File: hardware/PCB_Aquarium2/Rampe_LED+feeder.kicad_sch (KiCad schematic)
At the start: 5 parts, among them J28 Conn_01x03, J29 Conn_01x03, J30 Conn_01x03, J31 Conn_01x03, J32 Conn_01x03

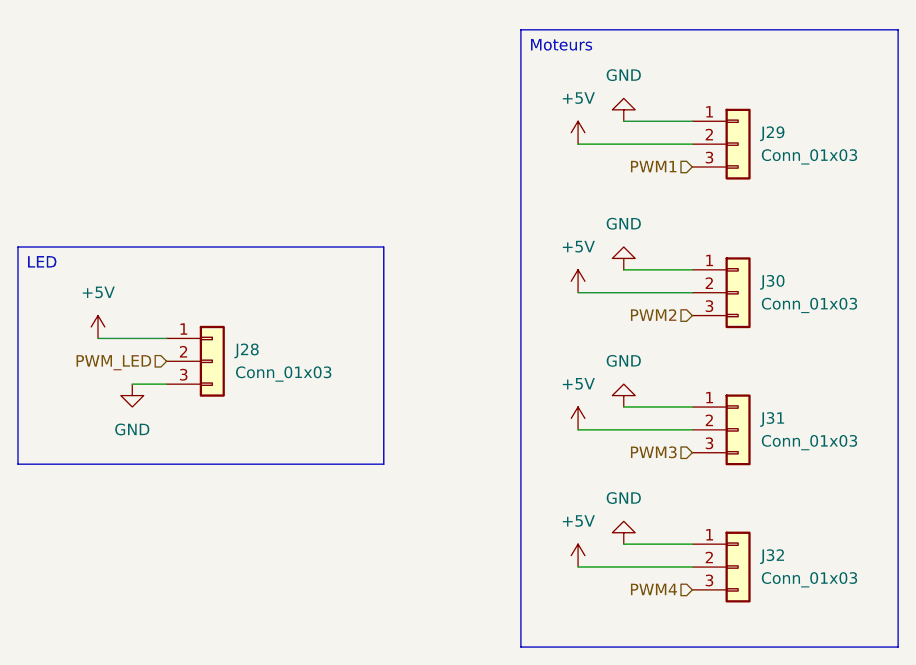
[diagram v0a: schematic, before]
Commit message: PCBs v3
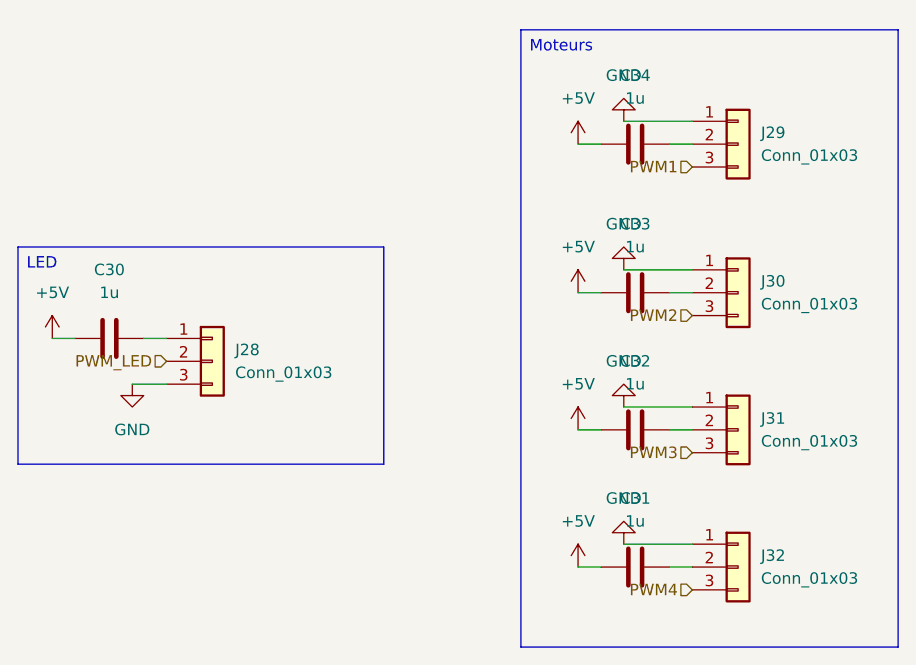
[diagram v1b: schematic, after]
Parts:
- added C30, C31, C32, C33, C34: 1u, Capacitor_SMD:C_0603_1608Metric, symbol Device:C
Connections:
- net +5V: now also C30.1, C31.1, C32.1, C33.1, C34.1; no longer J28.1 (Pin_1), J29.2 (Pin_2), J30.2 (Pin_2), J31.2 (Pin_2), J32.2 (Pin_2)
- new net: C33.2, J30.2 (Pin_2)
- new net: C30.2, J28.1 (Pin_1)
- new net: C31.2, J32.2 (Pin_2)
- new net: C32.2, J31.2 (Pin_2)
- new net: C34.2, J29.2 (Pin_2)

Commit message: PCBs v4
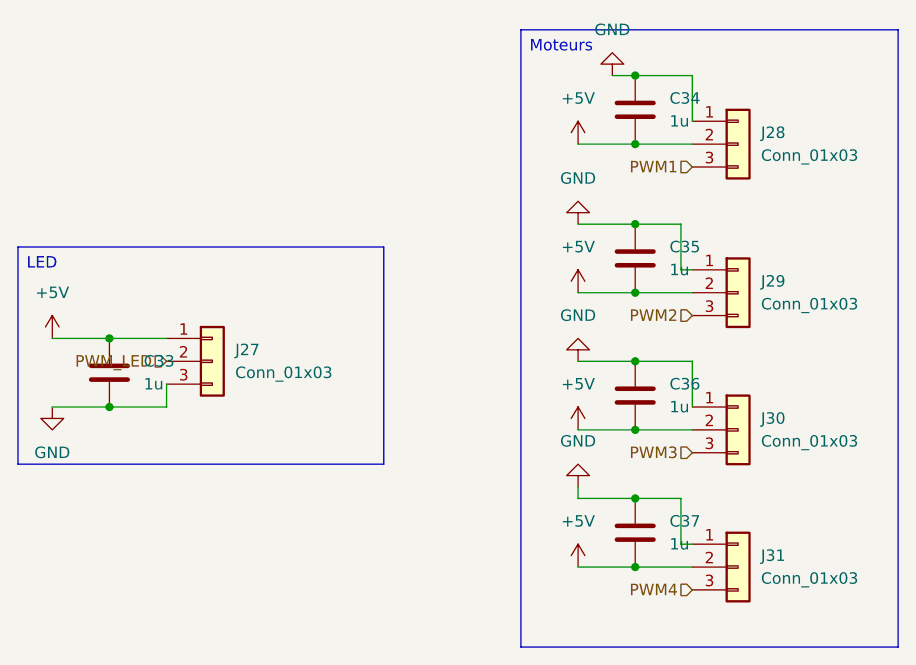
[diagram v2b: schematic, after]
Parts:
- renumbered C30 to C33, C33 to C35, C32 to C36, C31 to C37, J28 to J27, J29 to J28, J30 to J29, J31 to J30, J32 to J31
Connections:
- net +5V: now also C33.2, J27.1 (Pin_1), J28.2 (Pin_2), J29.2 (Pin_2), J30.2 (Pin_2), J31.2 (Pin_2); no longer C33.1
- net GND: now also C33.1, C34.2, C35.2, C36.2, C37.2
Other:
- moved on the sheet: C33, C34, C35, C36, C37
